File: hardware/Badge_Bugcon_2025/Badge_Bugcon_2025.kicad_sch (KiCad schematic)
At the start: 0 parts

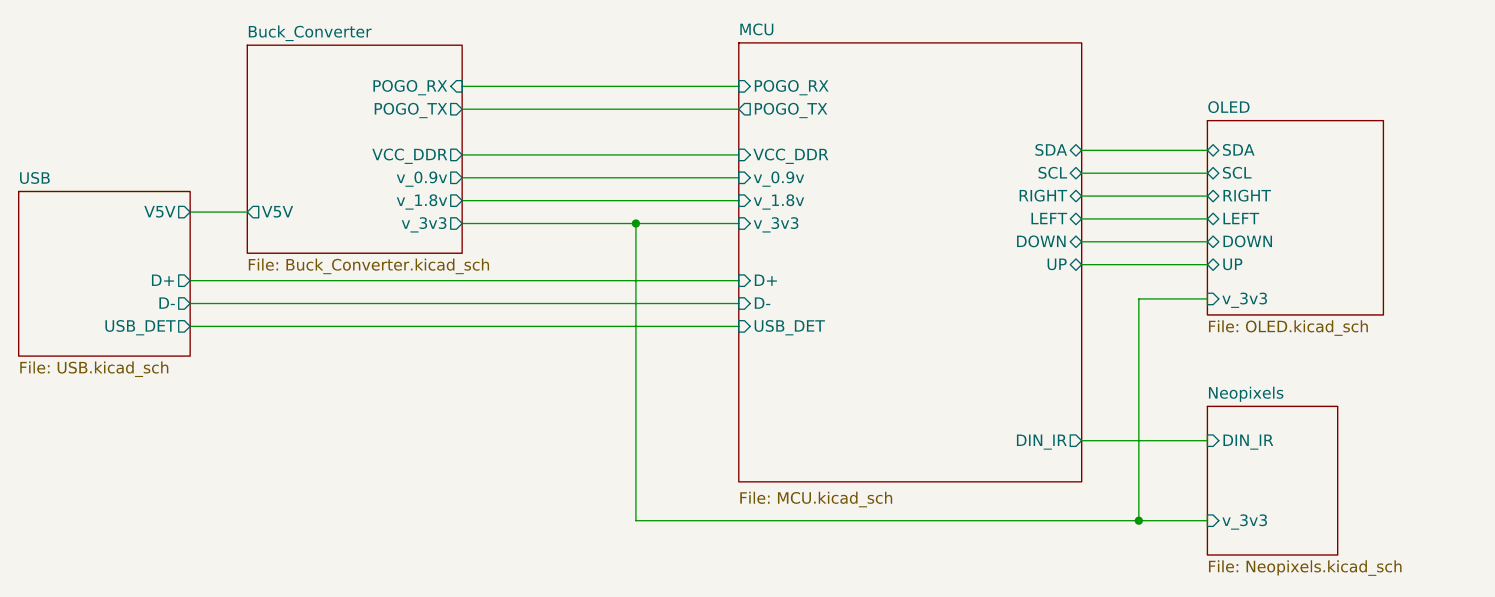
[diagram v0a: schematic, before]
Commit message: feat(Hw):Update_Schematic
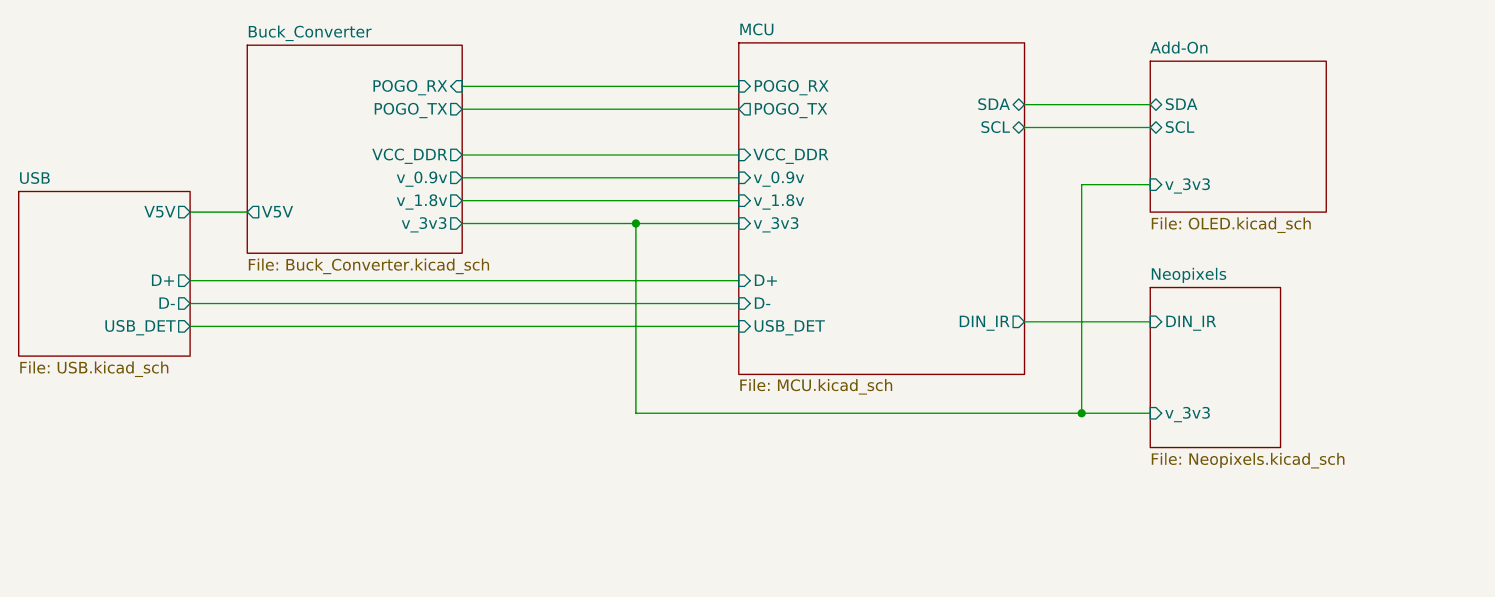
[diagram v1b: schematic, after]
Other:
- sheet OLED renamed Add-On
- sheet Add-On ports: added none; removed DOWN, LEFT, RIGHT, UP
- sheet MCU ports: added none; removed DOWN, LEFT, RIGHT, UP
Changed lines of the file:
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@@
 	(paper "A4")
 	(junction
-		(at 185.42 116.078)
+		(at 179.07 104.14)
 		(diameter 0)
 		(color 255 23 32 1)
@@
 	(wire
 		(pts
-			(xy 129.54 83.058) (xy 129.54 116.078)
+			(xy 129.54 83.058) (xy 129.54 104.14)
 		)
 		(stroke
@@
 	(wire
 		(pts
-			(xy 179.07 77.47) (xy 193.04 77.47)
+			(xy 172.72 72.39) (xy 186.69 72.39)
 		)
 		(stroke
@@
 	(wire
 		(pts
-			(xy 179.07 82.55) (xy 193.04 82.55)
-		)
-		(stroke
-			(width 0)
-			(type default)
-		)
-	)
-	(wire
-		(pts
-			(xy 185.42 91.44) (xy 185.42 116.078)
+			(xy 179.07 78.74) (xy 179.07 104.14)
 		)
 		(stroke
@@
 	(wire
 		(pts
-			(xy 185.42 91.44) (xy 193.04 91.44)
+			(xy 179.07 78.74) (xy 186.69 78.74)
 		)
 		(stroke
@@
 	(wire
 		(pts
-			(xy 179.07 107.188) (xy 193.04 107.188)
+			(xy 172.72 93.98) (xy 186.69 93.98)
 		)
 		(stroke
@@
 	(wire
 		(pts
-			(xy 179.07 80.01) (xy 193.04 80.01)
-		)
-		(stroke
-			(width 0)
-			(type default)
-		)
-	)
-	(wire
-		(pts
-			(xy 179.07 85.09) (xy 193.04 85.09)
-		)
-		(stroke
-			(width 0)
-			(type default)
-		)
-	)
-	(wire
-		(pts
-			(xy 179.07 87.63) (xy 193.04 87.63)
-		)
-		(stroke
-			(width 0)
-			(type default)
-		)
-	)
-	(wire
-		(pts
 			(xy 80.01 89.408) (xy 140.97 89.408)
 		)
@@
 	(wire
 		(pts
-			(xy 185.42 116.078) (xy 193.04 116.078)
+			(xy 179.07 104.14) (xy 186.69 104.14)
 		)
 		(stroke
@@
 	(wire
 		(pts
-			(xy 179.07 74.93) (xy 193.04 74.93)
-		)
-		(stroke
-			(width 0)
-			(type default)
-		)
-	)
-	(wire
-		(pts
-			(xy 129.54 116.078) (xy 185.42 116.078)
+			(xy 172.72 69.85) (xy 186.69 69.85)
+		)
+		(stroke
+			(width 0)
+			(type default)
+		)
+	)
+	(wire
+		(pts
+			(xy 129.54 104.14) (xy 179.07 104.14)
 		)
 		(stroke
@@
 	)
 	(sheet
-		(at 193.04 71.628)
-		(size 19.558 21.59)
+		(at 186.69 65.024)
+		(size 19.558 16.764)
 		(exclude_from_sim no)
 		(in_bom yes)
@@
 			(color 0 0 0 0.0000)
 		)
-		(property "Sheetname" "OLED"
-			(at 193.04 70.9164 0)
+		(property "Sheetname" "Add-On"
+			(at 186.69 64.3124 0)
 			(effects
 				(font
@@
 		)
 		(property "Sheetfile" "OLED.kicad_sch"
-			(at 193.04 93.8026 0)
+			(at 186.69 82.3726 0)
 			(effects
 				(font
@@
 			)
 		)
-		(pin "DOWN" bidirectional
-			(at 193.04 85.09 180)
-			(effects
-				(font
-					(size 1.27 1.27)
-				)
-				(justify left)
-			)
-		)
-		(pin "LEFT" bidirectional
-			(at 193.04 82.55 180)
-			(effects
-				(font
-					(size 1.27 1.27)
-				)
-				(justify left)
-			)
-		)
-		(pin "RIGHT" bidirectional
-			(at 193.04 80.01 180)
-			(effects
-				(font
-					(size 1.27 1.27)
-				)
-				(justify left)
-			)
-		)
 		(pin "SCL" bidirectional
-			(at 193.04 77.47 180)
+			(at 186.69 72.39 180)
 			(effects
 				(font
@@
 		)
 		(pin "SDA" bidirectional
-			(at 193.04 74.93 180)
-			(effects
-				(font
-					(size 1.27 1.27)
-				)
-				(justify left)
-			)
-		)
-		(pin "UP" bidirectional
-			(at 193.04 87.63 180)
+			(at 186.69 69.85 180)
 			(effects
 				(font
@@
 		)
 		(pin "v_3v3" input
-			(at 193.04 91.44 180)
+			(at 186.69 78.74 180)
 			(effects
 				(font
@@
 	)
 	(sheet
-		(at 193.04 103.378)
-		(size 14.478 16.51)
+		(at 186.69 90.17)
+		(size 14.478 17.78)
 		(exclude_from_sim no)
 		(in_bom yes)
@@
 		)
 		(property "Sheetname" "Neopixels"
-			(at 193.04 102.6664 0)
+			(at 186.69 89.4584 0)
 			(effects
 				(font
@@
 		)
 		(property "Sheetfile" "Neopixels.kicad_sch"
-			(at 193.04 120.4726 0)
+			(at 186.69 108.5346 0)
 			(effects
 				(font
@@
 		)
 		(pin "DIN_IR" input
-			(at 193.04 107.188 180)
+			(at 186.69 93.98 180)
 			(effects
 				(font
@@
 		)
 		(pin "v_3v3" input
-			(at 193.04 116.078 180)
+			(at 186.69 104.14 180)
 			(effects
 				(font
@@
 	(sheet
 		(at 140.97 62.992)
-		(size 38.1 48.768)
+		(size 31.75 36.83)
 		(exclude_from_sim no)
 		(in_bom yes)
@@
 		)
 		(property "Sheetfile" "MCU.kicad_sch"
-			(at 140.97 112.8526 0)
+			(at 140.97 100.33 0)
 			(effects
 				(font
@@
 		)
 		(pin "DIN_IR" output
-			(at 179.07 107.188 0)
-			(effects
-				(font
-					(size 1.27 1.27)
-				)
-				(justify right)
-			)
-		)
-		(pin "DOWN" bidirectional
-			(at 179.07 85.09 0)
-			(effects
-				(font
-					(size 1.27 1.27)
-				)
-				(justify right)
-			)
-		)
-		(pin "LEFT" bidirectional
-			(at 179.07 82.55 0)
-			(effects
-				(font
-					(size 1.27 1.27)
-				)
-				(justify right)
-			)
-		)
-		(pin "RIGHT" bidirectional
-			(at 179.07 80.01 0)
+			(at 172.72 93.98 0)
 			(effects
 				(font
@@
 		)
 		(pin "SCL" bidirectional
-			(at 179.07 77.47 0)
+			(at 172.72 72.39 0)
 			(effects
 				(font
@@
 		)
 		(pin "SDA" bidirectional
-			(at 179.07 74.93 0)
-			(effects
-				(font
-					(size 1.27 1.27)
-				)
-				(justify right)
-			)
-		)
-		(pin "UP" bidirectional
-			(at 179.07 87.63 0)
-			(effects
-				(font
+			(at 172.72 69.85 0)
+			(effects
+				(font
